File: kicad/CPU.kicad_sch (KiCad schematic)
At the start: 7 parts

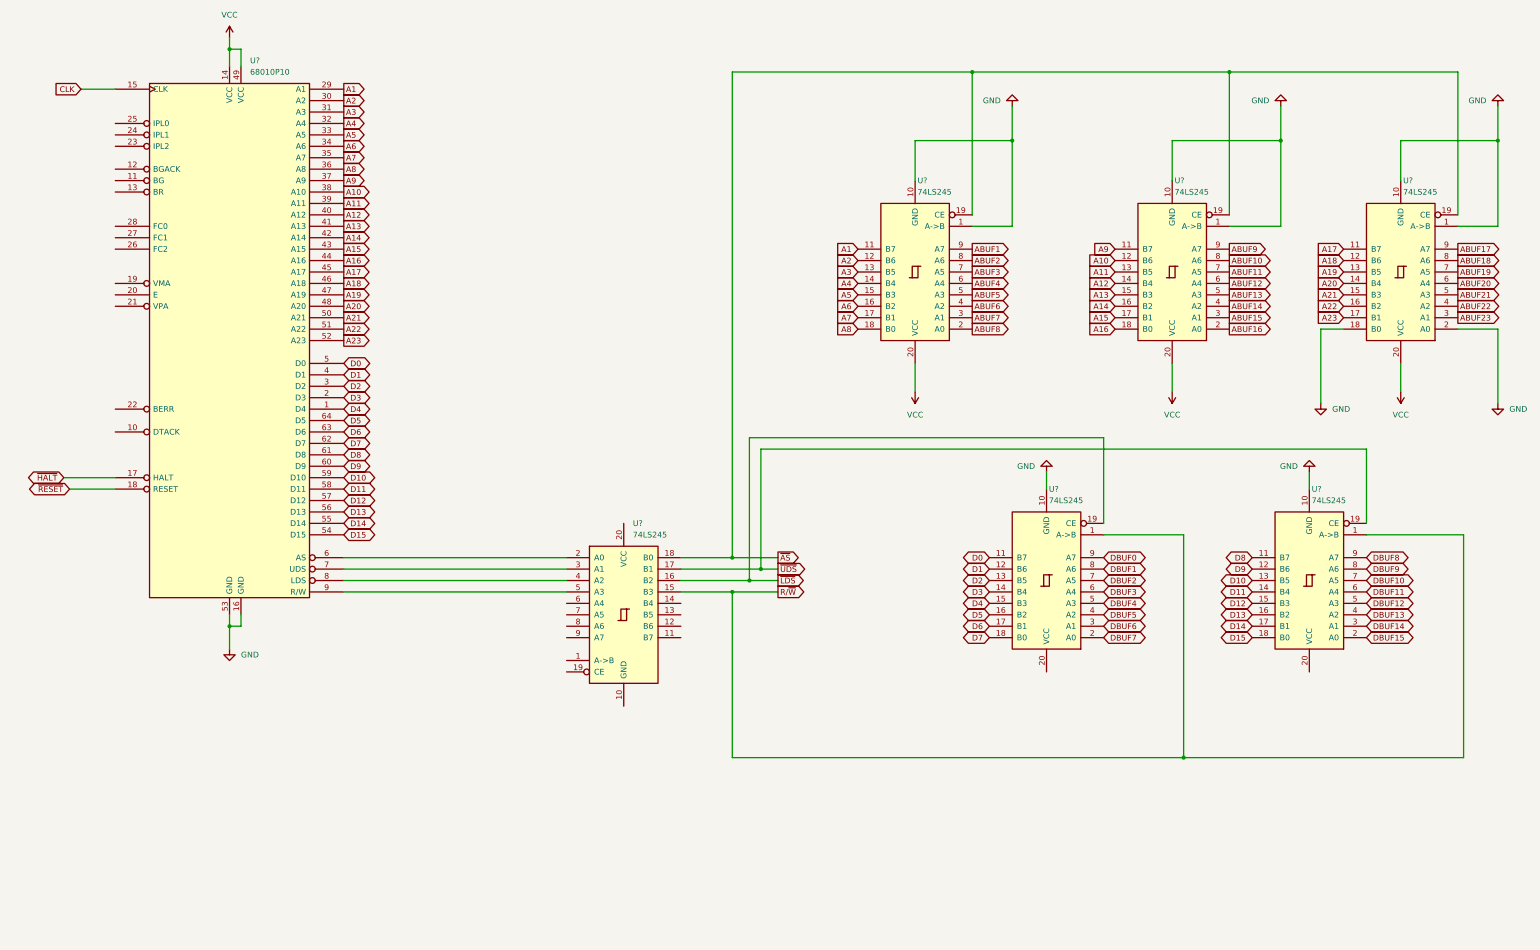
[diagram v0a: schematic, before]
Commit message: KiCad updates
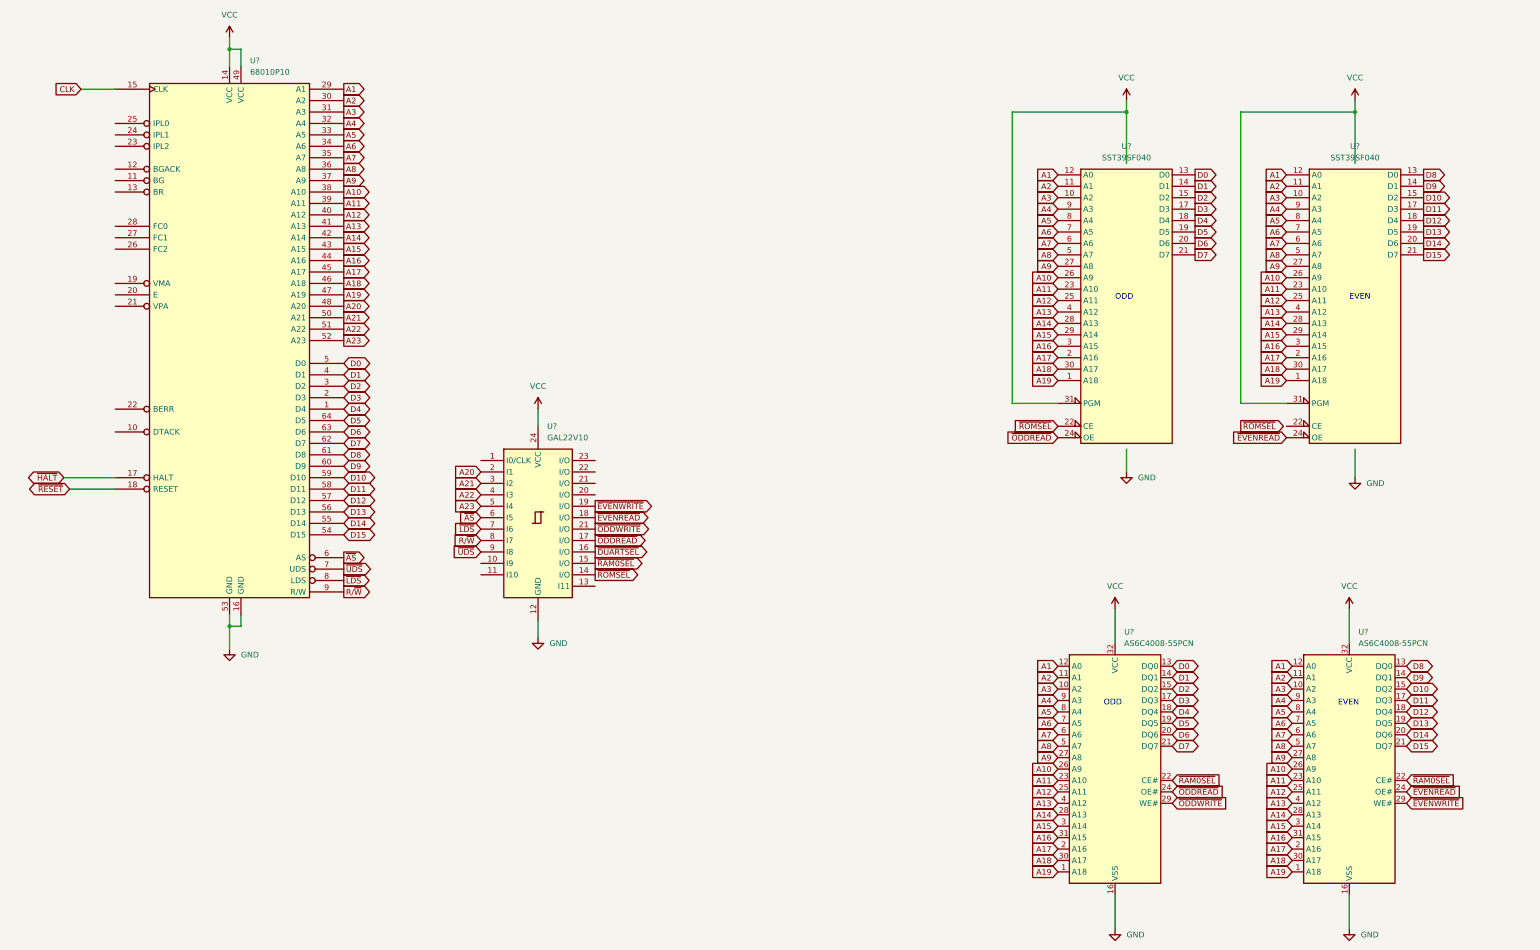
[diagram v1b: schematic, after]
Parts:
- removed U? (x6): 74LS245, symbol 74xx:74LS245
- added U? (x2): AS6C4008-55PCN, Package_DIP:DIP-32_W15.24mm, symbol Memory_RAM:AS6C4008-55PCN
- added U? (x2): SST39SF040, symbol Memory_Flash:SST39SF040
- added U?: GAL22V10, symbol Lattice_GAL_sym:GAL22V10
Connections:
- net A1: now also U?.12 (A0), U?.12 (A0), U?.12 (A0), U?.12 (A0)
- net A10: now also U?.26 (A9), U?.26 (A9), U?.26 (A9), U?.26 (A9)
- net A11: now also U?.23 (A10), U?.23 (A10), U?.23 (A10), U?.23 (A10)
- net A12: now also U?.25 (A11), U?.25 (A11), U?.25 (A11), U?.25 (A11)
- net A13: now also U?.4 (A12), U?.4 (A12), U?.4 (A12), U?.4 (A12)
- net A14: now also U?.28 (A13), U?.28 (A13), U?.28 (A13), U?.28 (A13)
- net A15: now also U?.29 (A14), U?.29 (A14), U?.3 (A14), U?.3 (A14)
- net A16: now also U?.3 (A15), U?.3 (A15), U?.31 (A15), U?.31 (A15)
- net A17: now also U?.2 (A16), U?.2 (A16), U?.2 (A16), U?.2 (A16)
- net A18: now also U?.30 (A17), U?.30 (A17), U?.30 (A17), U?.30 (A17)
- net A19: now also U?.1 (A18), U?.1 (A18), U?.1 (A18), U?.1 (A18)
- net A2: now also U?.11 (A1), U?.11 (A1), U?.11 (A1), U?.11 (A1)
- net A20: now also U?.2 (I1)
- net A21: now also U?.3 (I2)
- net A22: now also U?.4 (I3)
- net A23: now also U?.5 (I4)
- net A3: now also U?.10 (A2), U?.10 (A2), U?.10 (A2), U?.10 (A2)
- net A4: now also U?.9 (A3), U?.9 (A3), U?.9 (A3), U?.9 (A3)
- net A5: now also U?.8 (A4), U?.8 (A4), U?.8 (A4), U?.8 (A4)
- net A6: now also U?.7 (A5), U?.7 (A5), U?.7 (A5), U?.7 (A5)
- net A7: now also U?.6 (A6), U?.6 (A6), U?.6 (A6), U?.6 (A6)
- net A8: now also U?.5 (A7), U?.5 (A7), U?.5 (A7), U?.5 (A7)
- net A9: now also U?.27 (A8), U?.27 (A8), U?.27 (A8), U?.27 (A8)
- net D0: now also U?.13 (D0), U?.13 (DQ0)
- net D1: now also U?.14 (D1), U?.14 (DQ1)
- net D10: now also U?.15 (D2), U?.15 (DQ2)
- net D11: now also U?.17 (D3), U?.17 (DQ3)
- net D12: now also U?.18 (D4), U?.18 (DQ4)
- net D13: now also U?.19 (D5), U?.19 (DQ5)
- net D14: now also U?.20 (D6), U?.20 (DQ6)
- net D15: now also U?.21 (D7), U?.21 (DQ7)
- net D2: now also U?.15 (D2), U?.15 (DQ2)
- net D3: now also U?.17 (D3), U?.17 (DQ3)
- net D4: now also U?.18 (D4), U?.18 (DQ4)
- net D5: now also U?.19 (D5), U?.19 (DQ5)
- net D6: now also U?.20 (D6), U?.20 (DQ6)
- net D7: now also U?.21 (D7), U?.21 (DQ7)
- net D8: now also U?.13 (D0), U?.13 (DQ0)
- net D9: now also U?.14 (D1), U?.14 (DQ1)
- net GND: now also U?.12 (GND), U?.16 (GND), U?.16 (GND), U?.16 (VSS), U?.16 (VSS)
- net R/~{W}: now also U?.9 (R/W), U?.8 (I7)
- net VCC: now also U?.24 (VCC), U?.31 (PGM), U?.31 (PGM), U?.32 (VCC), U?.32 (VCC), U?.32 (VCC), U?.32 (VCC)
- net ~{AS}: now also U?.6 (AS), U?.6 (I5)
- net ~{LDS}: now also U?.8 (LDS), U?.7 (I6)
- net ~{UDS}: now also U?.7 (UDS), U?.9 (I8)
- new net ~{DUARTSEL}: U?.16 (I/O)
- new net ~{EVENREAD}: U?.18 (I/O), U?.24 (OE#), U?.24 (OE)
- new net ~{EVENWRITE}: U?.19 (I/O), U?.29 (WE#)
- new net ~{ODDREAD}: U?.17 (I/O), U?.24 (OE#), U?.24 (OE)
- new net ~{ODDWRITE}: U?.21 (I/O), U?.29 (WE#)
- new net ~{RAM0SEL}: U?.15 (I/O), U?.22 (CE#), U?.22 (CE#)
- new net ~{ROMSEL}: U?.14 (I/O), U?.22 (CE)
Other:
- note added: "EVEN"
- note added: "ODD"
